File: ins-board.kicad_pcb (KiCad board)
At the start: 4 copper layers, 50 x 23 mm, 94 parts, among them P1 PWR, P2 Power (Solder Pad), Q1 FDN306P, Q2 FDC638APZ, U1 24LC128, U10 HMC5883L, U11 H3LIS331DL, U2 STM32F415RGT6, U3 LTC4412, U4 MAX3051, U5 LT1965, U6 LT1761-3.3, U7 LT1965, U8 MS5611-01BA, U9 MPU6000, X1 CRYSTAL 16MHz 10ppm

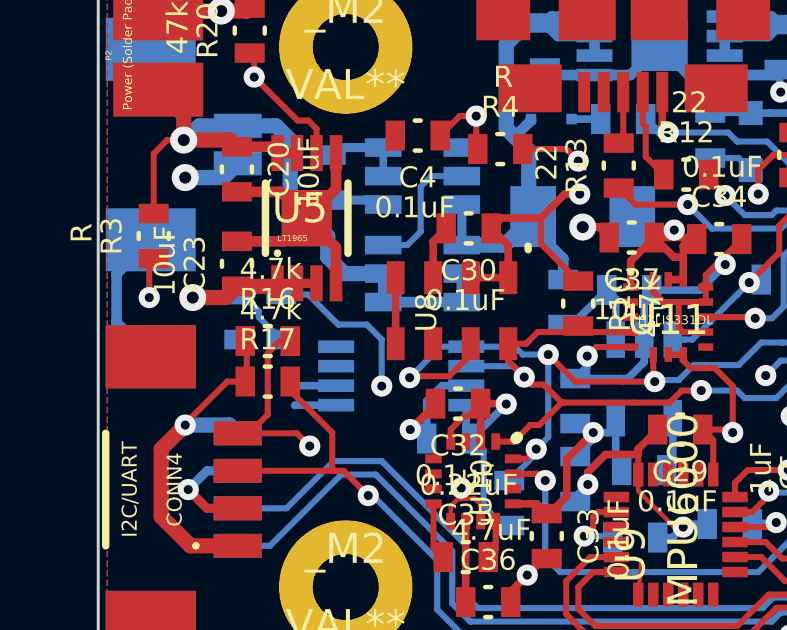
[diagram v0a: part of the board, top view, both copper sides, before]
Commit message: optimize routing
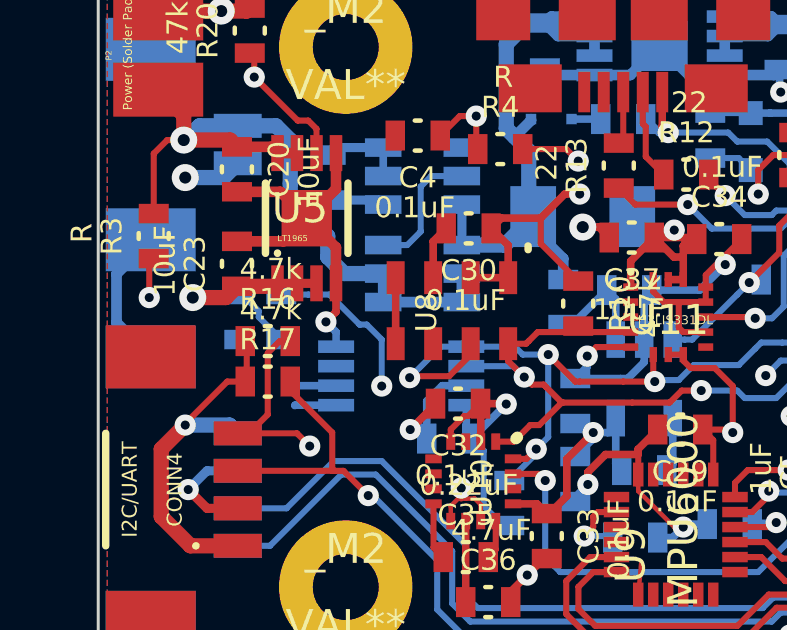
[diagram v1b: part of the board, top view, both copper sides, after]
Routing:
- net GND: track 140.3 -> 142.7 mm, vias 25 -> 26
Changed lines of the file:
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@@
     (thickness 1.6)
     (drawings 13)
-    (tracks 1273)
+    (tracks 1281)
     (zones 0)
     (modules 94)
@@
   (segment (start 45.6646 38.5646) (end 45.6646 38.3872) (width 0.2032) (layer F.Cu) (net 28))
   (segment (start 45.6646 38.3872) (end 45.6646 38.5646) (width 0.2032) (layer F.Cu) (net 28))
-  (segment (start 44.4146 38.3872) (end 44.4146 38.7554) (width 0.2032) (layer F.Cu) (net 29) (status C00000))
-  (segment (start 43.4132 38.4868) (end 44.2698 38.4868) (width 0.2032) (layer B.Cu) (net 29) (status 800000))
+  (segment (start 44.4146 38.3872) (end 44.4146 38.7554) (width 0.2032) (layer F.Cu) (net 29))
+  (segment (start 43.4132 38.4868) (end 44.2698 38.4868) (width 0.2032) (layer B.Cu) (net 29))
   (segment (start 42.38 39.52) (end 43.4132 38.4868) (width 0.2032) (layer B.Cu) (net 29))
   (via (at 42.38 39.52) (size 0.706) (layers F.Cu B.Cu) (net 29))
   (segment (start 42.43 39.47) (end 42.38 39.52) (width 0.2032) (layer F.Cu) (net 29))
   (segment (start 43.7 39.47) (end 42.43 39.47) (width 0.2032) (layer F.Cu) (net 29))
-  (segment (start 44.4146 38.7554) (end 43.7 39.47) (width 0.2032) (layer F.Cu) (net 29) (status 400000))
+  (segment (start 44.4146 38.7554) (end 43.7 39.47) (width 0.2032) (layer F.Cu) (net 29))
   (segment (start 46.6 41.9) (end 46.6 42.05) (width 0.2032) (layer B.Cu) (net 29))
   (segment (start 46.6 42.05) (end 45.7 42.95) (width 0.2032) (layer B.Cu) (net 29))
@@
   (segment (start 61.4 44.4) (end 59.8 46) (width 0.2032) (layer F.Cu) (net 35))
   (segment (start 48.5 45.5) (end 49.275 45.5) (width 0.2032) (layer F.Cu) (net 35))
-  (segment (start 46.95 44.05) (end 47.04 44.05) (width 0.254) (layer F.Cu) (net 36) (status C00000))
+  (segment (start 46.95 44.05) (end 47.04 44.05) (width 0.254) (layer F.Cu) (net 36))
   (segment (start 47.62 42.23) (end 48.5 41.35) (width 0.254) (layer F.Cu) (net 36))
   (segment (start 47.62 43.47) (end 47.62 42.23) (width 0.254) (layer F.Cu) (net 36))
-  (segment (start 47.04 44.05) (end 47.62 43.47) (width 0.254) (layer F.Cu) (net 36) (status 400000))
+  (segment (start 47.04 44.05) (end 47.62 43.47) (width 0.254) (layer F.Cu) (net 36))
   (segment (start 46.75 34.2) (end 46.75 35.05) (width 0.2032) (layer F.Cu) (net 36))
   (segment (start 46.75 35.05) (end 48 36.3) (width 0.2032) (layer F.Cu) (net 36))
@@
   (segment (start 66.25 38.75) (end 66 39) (width 0.2032) (layer F.Cu) (net 51))
   (segment (start 66.25 38.75) (end 66 39) (width 0.2032) (layer F.Cu) (net 51))
+  (segment (start 39.925 36.375) (end 39.925 37.325) (width 0.254) (layer F.Cu) (net 52) (status 400000))
+  (segment (start 39.9288 37.9988) (end 39.9288 38.4868) (width 0.254) (layer B.Cu) (net 52) (status 800000))
+  (segment (start 39.59 37.66) (end 39.9288 37.9988) (width 0.254) (layer B.Cu) (net 52))
+  (via (at 39.59 37.66) (size 0.706) (layers F.Cu B.Cu) (net 52))
+  (segment (start 39.925 37.325) (end 39.59 37.66) (width 0.254) (layer F.Cu) (net 52))
   (segment (start 49.99 42.08) (end 49.99 41.91) (width 0.254) (layer F.Cu) (net 52))
-  (segment (start 49.99 41.91) (end 50.65 41.25) (width 0.254) (layer F.Cu) (net 52) (status 800000))
-  (segment (start 47.9 43.65) (end 47.9 43.5) (width 0.254) (layer B.Cu) (net 52) (status C00000))
+  (segment (start 49.99 41.91) (end 50.65 41.25) (width 0.254) (layer F.Cu) (net 52))
+  (segment (start 47.9 43.65) (end 47.9 43.5) (width 0.254) (layer B.Cu) (net 52))
   (segment (start 48.91 42.08) (end 49.99 42.08) (width 0.254) (layer F.Cu) (net 52))
   (segment (start 49.99 42.08) (end 50 42.08) (width 0.254) (layer F.Cu) (net 52))
@@
   (segment (start 48.32 43.08) (end 48.32 42.67) (width 0.254) (layer F.Cu) (net 52))
   (via (at 48.32 43.08) (size 0.706) (layers F.Cu B.Cu) (net 52))
-  (segment (start 47.9 43.5) (end 48.32 43.08) (width 0.254) (layer B.Cu) (net 52) (status 400000))
+  (segment (start 47.9 43.5) (end 48.32 43.08) (width 0.254) (layer B.Cu) (net 52))
   (segment (start 57.225 37.25) (end 55.78 37.25) (width 0.2032) (layer B.Cu) (net 52))
   (segment (start 55.6 37.07) (end 55.6 36.25) (width 0.2032) (layer B.Cu) (net 52))
@@
   (via (at 54.6 44.35) (size 0.706) (layers F.Cu B.Cu) (net 76))
   (segment (start 54.45 44.5) (end 54.6 44.35) (width 0.2032) (layer F.Cu) (net 76))
-  (segment (start 41.45 39.8) (end 41.45 33) (width 0.2032) (layer Inner2.Cu) (net 77))
-  (segment (start 41.45 33) (end 42.01 32.44) (width 0.2032) (layer Inner2.Cu) (net 77))
+  (segment (start 41.45 39.8) (end 41.45 39.25) (width 0.2032) (layer Inner2.Cu) (net 77))
+  (segment (start 42.55 38.15) (end 42.55 31.9) (width 0.2032) (layer Inner2.Cu) (net 77))
+  (segment (start 41.45 39.25) (end 42.55 38.15) (width 0.2032) (layer Inner2.Cu) (net 77))
+  (segment (start 40.73 37.75) (end 40.71 37.75) (width 0.2032) (layer B.Cu) (net 77))
+  (segment (start 39.71 36.75) (end 39 36.75) (width 0.2032) (layer B.Cu) (net 77))
+  (segment (start 40.71 37.75) (end 39.71 36.75) (width 0.2032) (layer B.Cu) (net 77))
   (segment (start 52.4 30.7) (end 53.75 30.7) (width 0.2032) (layer B.Cu) (net 77))
   (segment (start 53.75 30.7) (end 54.4 30.7) (width 0.254) (layer B.Cu) (net 77))
@@
   (via (at 41.45 39.8) (size 0.706) (layers F.Cu B.Cu) (net 77))
   (segment (start 39 36.75) (end 38.1 36.75) (width 0.2032) (layer B.Cu) (net 77))
-  (segment (start 40 37.75) (end 39 36.75) (width 0.2032) (layer B.Cu) (net 77))
-  (segment (start 40.95 37.75) (end 40 37.75) (width 0.2032) (layer B.Cu) (net 77))
+  (segment (start 40.95 37.75) (end 40.73 37.75) (width 0.2032) (layer B.Cu) (net 77))
   (segment (start 41.45 38.25) (end 40.95 37.75) (width 0.2032) (layer B.Cu) (net 77))
   (segment (start 74.25 35.9) (end 75.1 35.9) (width 0.254) (layer F.Cu) (net 77))
@@
   (segment (start 53.4 29.5) (end 54.05 28.85) (width 0.2032) (layer Inner2.Cu) (net 77))
   (segment (start 44.95 29.5) (end 53.4 29.5) (width 0.2032) (layer Inner2.Cu) (net 77))
-  (segment (start 42.01 32.44) (end 44.95 29.5) (width 0.2032) (layer Inner2.Cu) (net 77))
+  (segment (start 42.55 31.9) (end 44.95 29.5) (width 0.2032) (layer Inner2.Cu) (net 77))
   (segment (start 52.8828 28.1328) (end 54.3276 28.1328) (width 0.3556) (layer B.Cu) (net 77))
   (segment (start 54.3276 28.1328) (end 54.7116 27.7488) (width 0.3556) (layer B.Cu) (net 77))
